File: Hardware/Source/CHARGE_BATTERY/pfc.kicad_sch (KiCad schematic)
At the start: 2 parts, among them U1 UCC28180D

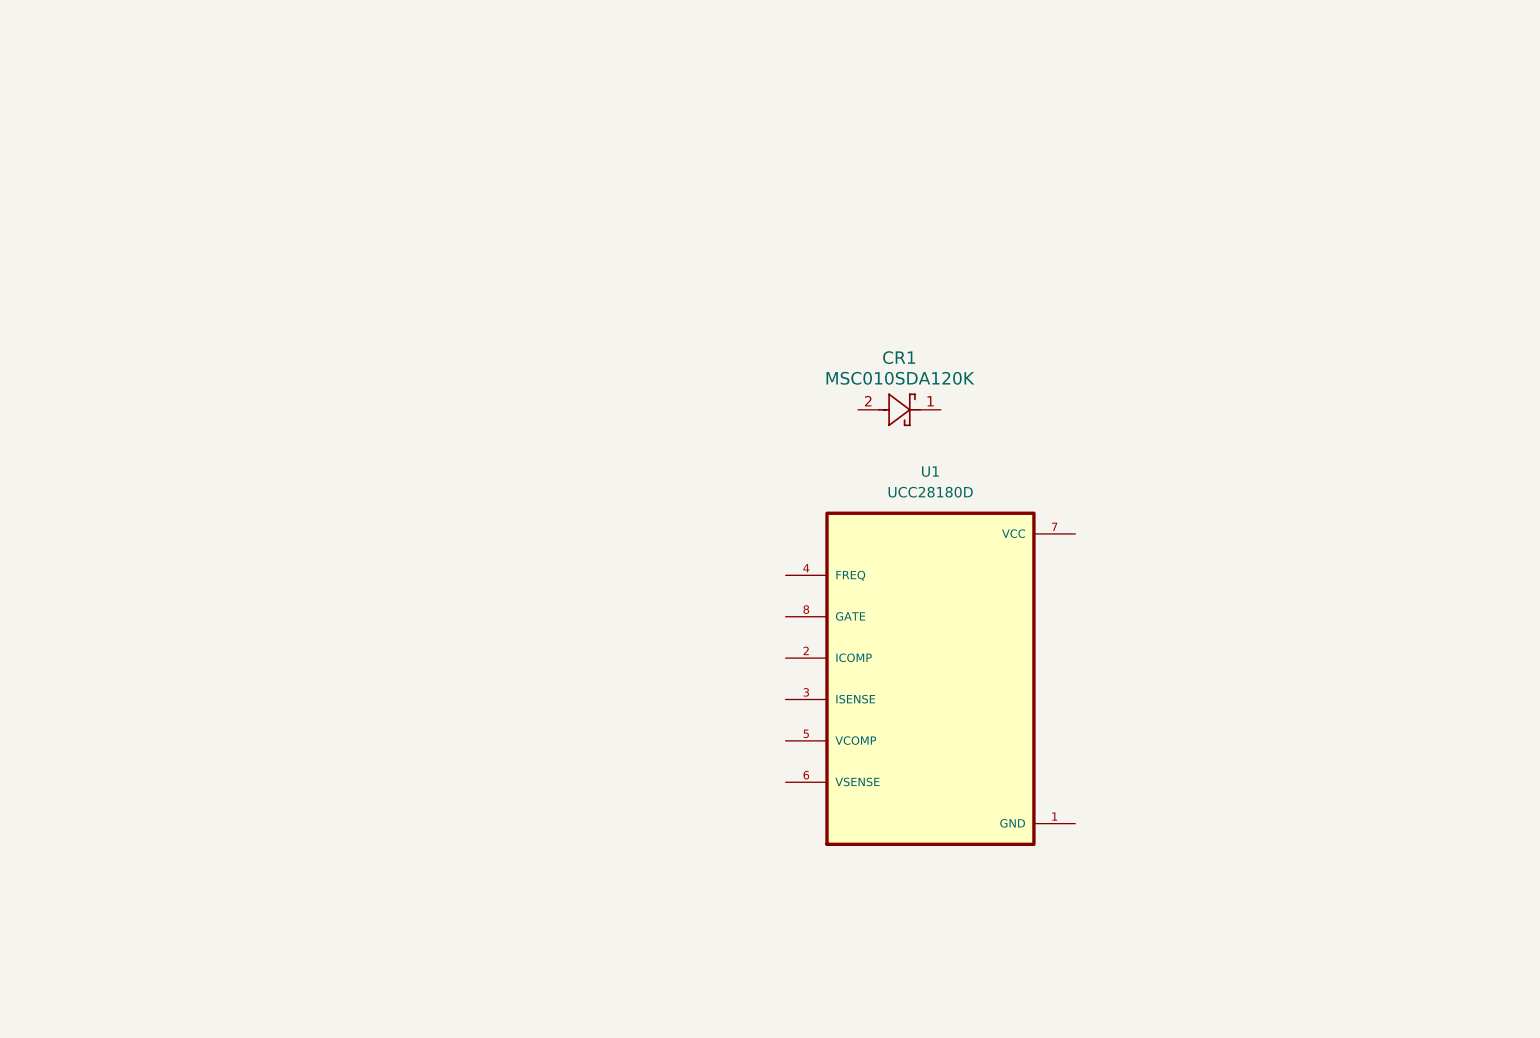
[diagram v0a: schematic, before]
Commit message: hardware:sche:update PFC
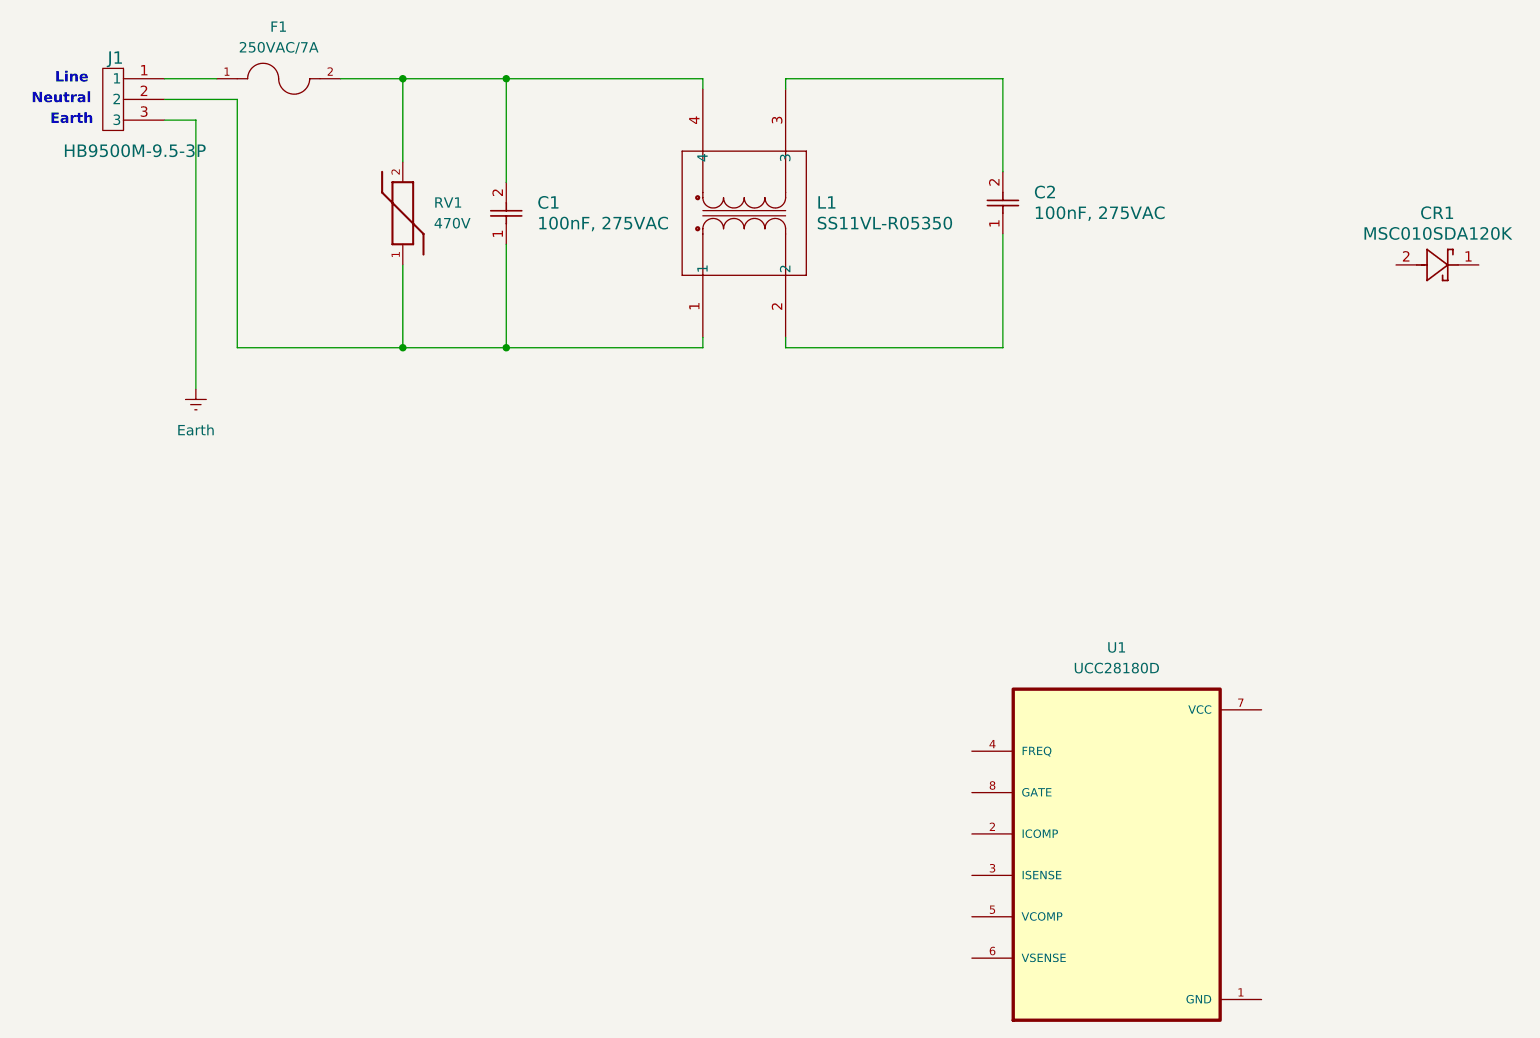
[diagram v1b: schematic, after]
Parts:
- added C1, C2: 100nF, 275VAC, charge_battery_footprint_lib:CAP_B32671P-10--5x11x13_TDK, symbol charge_battery_sym_lib:Film Cap
- added F1: 250VAC/7A, charge_battery_footprint_lib:FUSAD2722W65L2250D600, symbol charge_battery_sym_lib:FUSE_250VAC_7A
- added J1: HB9500M-9.5-3P, charge_battery_footprint_lib:CONN3_HB9500_KAN, symbol charge_battery_sym_lib:HB9500M-9.5-3P
- added L1: SS11VL-R05350, charge_battery_footprint_lib:IND_SS11VL-R05350_KEM, symbol charge_battery_sym_lib:SS11VL-R05350
- added RV1: 470V, charge_battery_footprint_lib:MOV07D471K, symbol charge_battery_sym_lib:MOV-07D471K
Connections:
- new net: C1.1, J1.2, L1.1, RV1.1
- new net: C1.2, F1.2, L1.4, RV1.2
- new net: C2.1, L1.2
- new net: C2.2, L1.3
- new net: F1.1, J1.1
- new net Earth: J1.3
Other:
- note added: "Earth"
- note added: "Line"
- note added: "Neutral"
- moved on the sheet: CR1, U1
